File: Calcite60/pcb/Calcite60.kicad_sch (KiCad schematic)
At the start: 56 parts, among them J1 USB_C_Receptacle_USB2.0, J2 Conn_01x02, J3 Conn_01x02, J4 Conn_01x02, J4 Conn_02x05_Counter_Clockwise, J5 Conn_01x02, J6 Conn_01x04, Q1 AO3407, SW1 SW_DPDT_x2, U1 SRV05-4, U2 TP4054, U3 RT9013-33GB

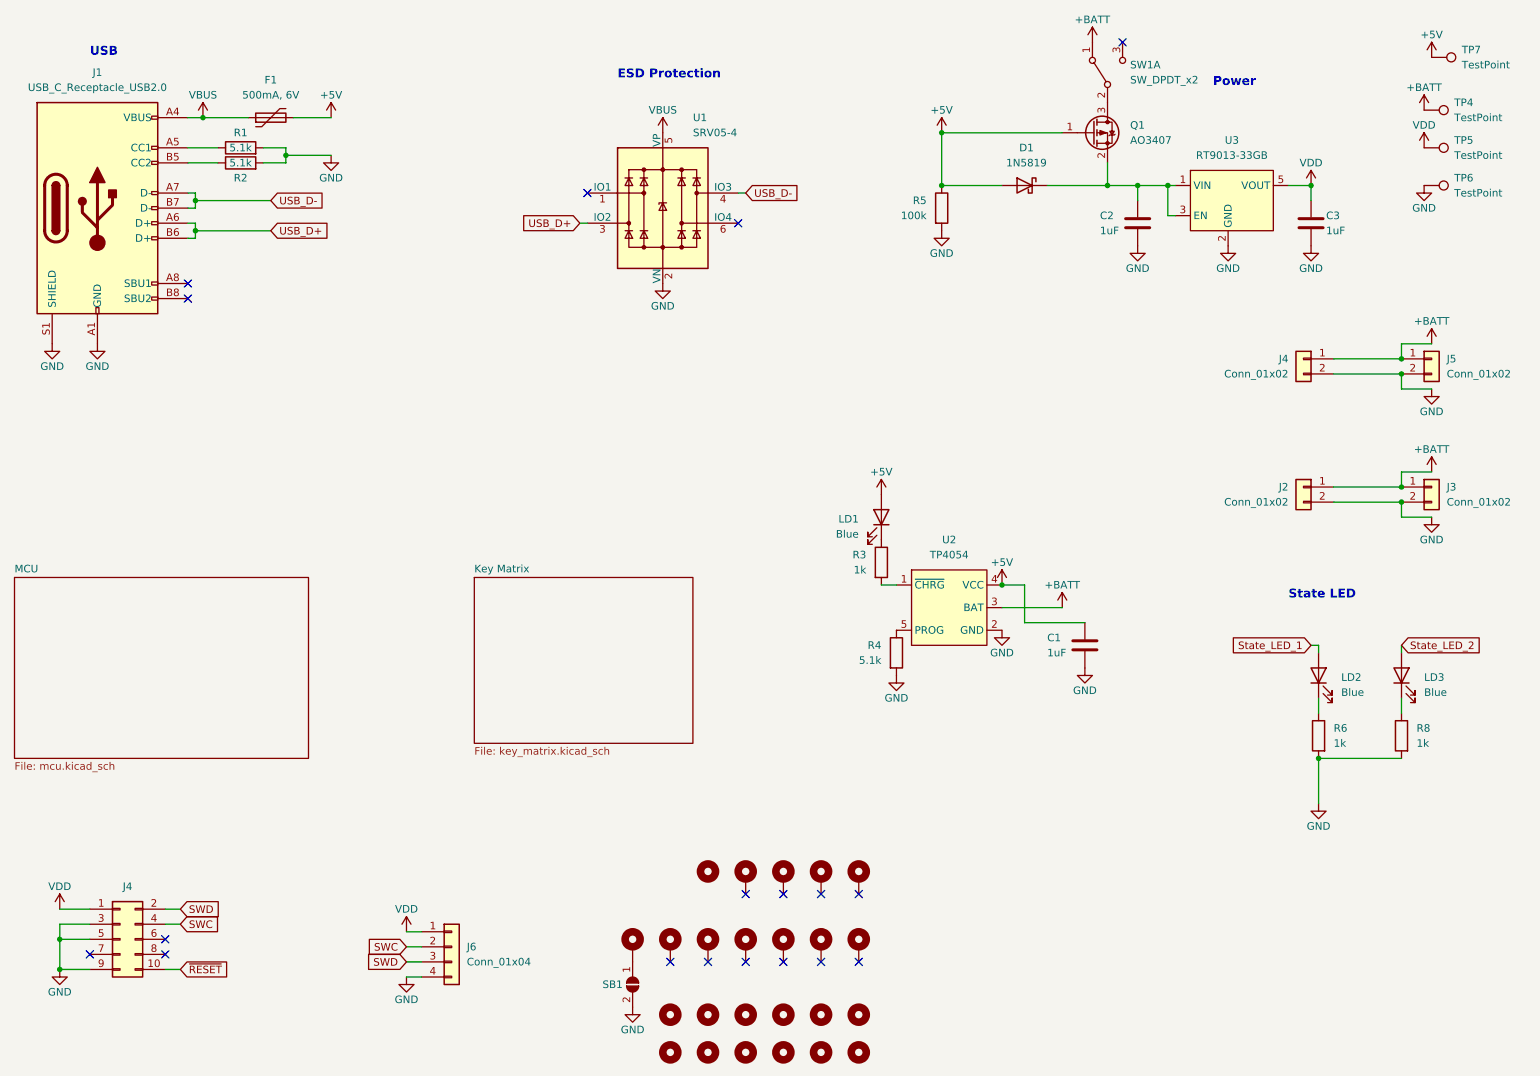
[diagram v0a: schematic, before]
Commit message: Update BOM
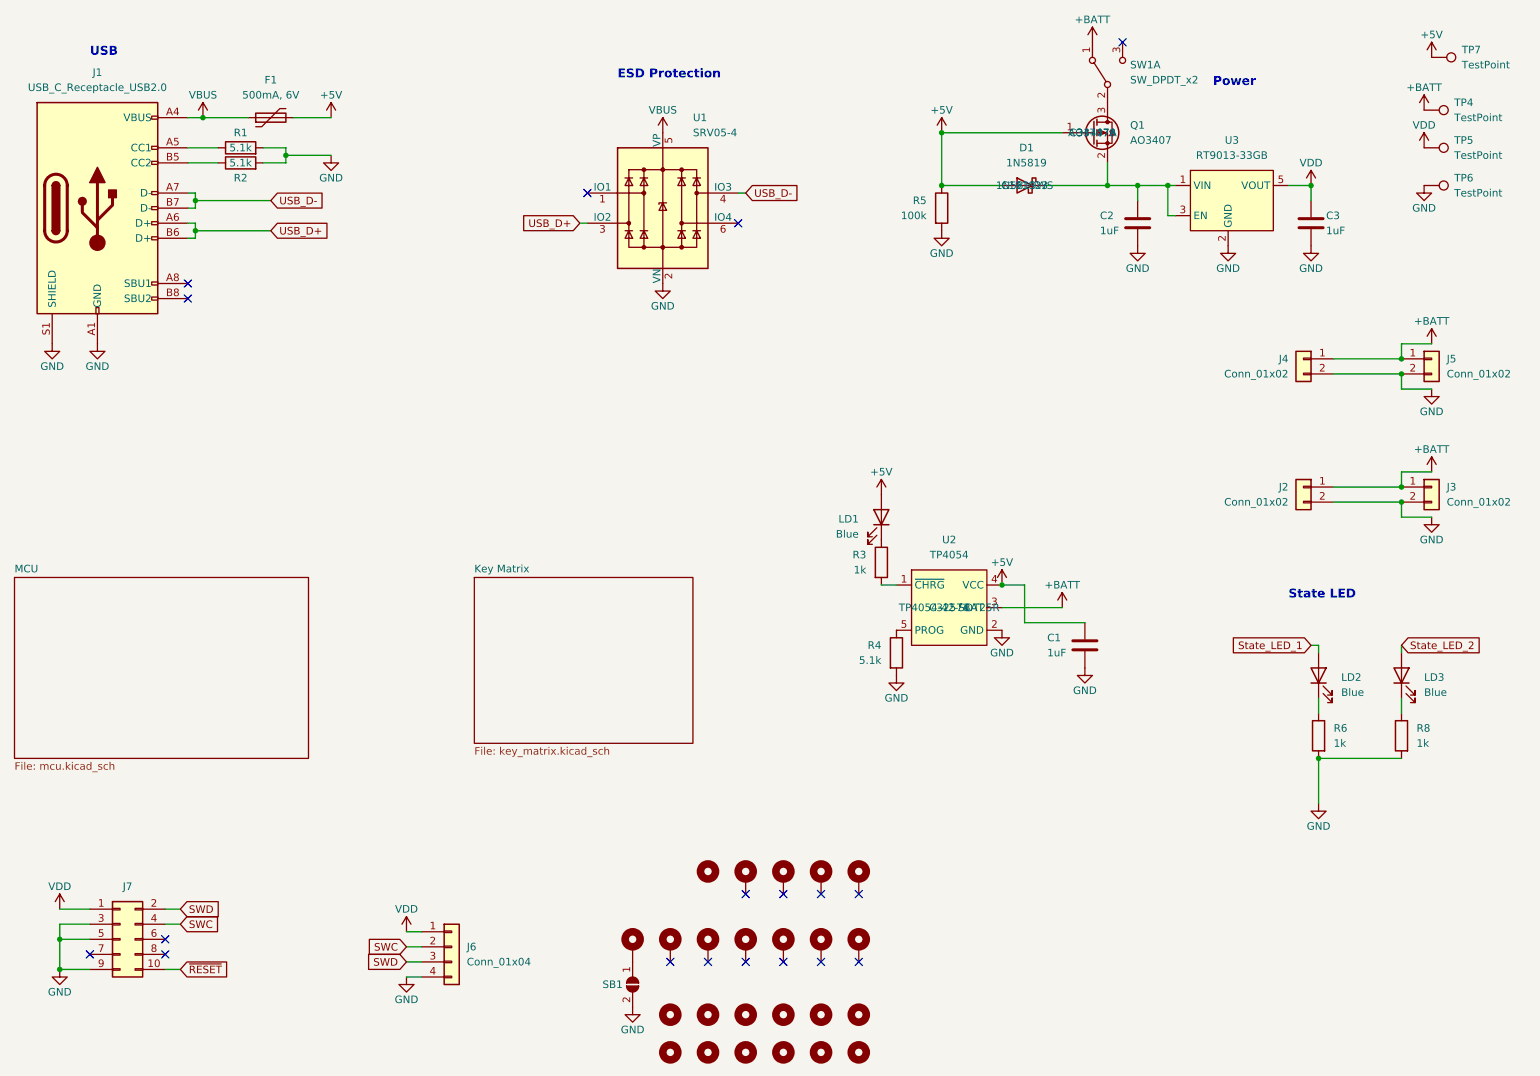
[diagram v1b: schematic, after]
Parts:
- C1, C2, C3: LCSC C52923 -> C15849; MFR. Part # CL05A105KA5NQNC -> CL10A105KB8NNNC
- D1: LCSC (none) -> C191023; MFR. Part # (none) -> 1N5819WS
- Q1: LCSC (none) -> C347478; MFR. Part # (none) -> AO3407A
- R1, R2: LCSC C25905 -> C23186; MFR. Part # 0402WGF5101TCE -> 0603WAF5101T5E
- R3, R6, R8: LCSC C11702 -> C21190; MFR. Part # 0402WGF1001TCE -> 0603WAF1001T5E
- R4: LCSC C11702 -> C23186; MFR. Part # 0402WGF1001TCE -> 0603WAF5101T5E
- R5: LCSC C11702 -> C25803; MFR. Part # 0402WGF1001TCE -> 0603WAF1003T5E
- U2: LCSC (none) -> C32574; MFR. Part # (none) -> TP4054-42-SOT25R
- renumbered J4 to J7
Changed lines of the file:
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@@
 (kicad_sch
-	(version 20231120)
+	(version 20250114)
 	(generator "eeschema")
-	(generator_version "8.0")
+	(generator_version "9.0")
 	(paper "A4")
 	(title_block
@@
 		(comment 2 "Kailh Choc V1 (PG1350) Low Profile Switches")
 	)
+	(text "ESD Protection"
+		(exclude_from_sim no)
+		(at 130.81 31.75 0)
+		(effects
+			(font
+				(size 1.5 1.5)
+				(thickness 0.3)
+				(bold yes)
+			)
+			(justify left bottom)
+		)
+	)
+	(text "State LED"
+		(exclude_from_sim no)
+		(at 243.84 119.38 0)
+		(effects
+			(font
+				(size 1.5 1.5)
+				(thickness 0.3)
+				(bold yes)
+			)
+			(justify left bottom)
+		)
+	)
+	(text "USB"
+		(exclude_from_sim no)
+		(at 41.91 27.94 0)
+		(effects
+			(font
+				(size 1.5 1.5)
+				(thickness 0.3)
+				(bold yes)
+			)
+			(justify left bottom)
+		)
+	)
+	(text "Power\n"
+		(exclude_from_sim no)
+		(at 231.14 33.02 0)
+		(effects
+			(font
+				(size 1.5 1.5)
+				(thickness 0.3)
+				(bold yes)
+			)
+			(justify left bottom)
+		)
+	)
 	(junction
 		(at 262.89 81.28)
@@
 		)
 	)
-	(text "ESD Protection"
-		(exclude_from_sim no)
-		(at 130.81 31.75 0)
-		(effects
-			(font
-				(size 1.5 1.5)
-				(thickness 0.3)
-				(bold yes)
-			)
-			(justify left bottom)
-		)
-	)
-	(text "State LED"
-		(exclude_from_sim no)
-		(at 243.84 119.38 0)
-		(effects
-			(font
-				(size 1.5 1.5)
-				(thickness 0.3)
-				(bold yes)
-			)
-			(justify left bottom)
-		)
-	)
-	(text "USB"
-		(exclude_from_sim no)
-		(at 41.91 27.94 0)
-		(effects
-			(font
-				(size 1.5 1.5)
-				(thickness 0.3)
-				(bold yes)
-			)
-			(justify left bottom)
-		)
-	)
-	(text "Power\n"
-		(exclude_from_sim no)
-		(at 231.14 33.02 0)
-		(effects
-			(font
-				(size 1.5 1.5)
-				(thickness 0.3)
-				(bold yes)
-			)
-			(justify left bottom)
-		)
-	)
 	(global_label "SWC"
 		(shape input)
@@
 			)
 		)
-		(property "MFR. Part #" "0402WGF1001TCE "
+		(property "MFR. Part #" "0603WAF1001T5E"
 			(at 262.89 142.24 0)
 			(effects
@@
 			)
 		)
-		(property "LCSC" "C11702"
+		(property "LCSC" "C21190"
 			(at 262.89 142.24 0)
 			(effects
@@
 			)
 		)
-		(property "MFR. Part #" "0402WGF1001TCE "
+		(property "MFR. Part #" "0603WAF5101T5E"
 			(at 177.8 128.27 0)
 			(effects
@@
 			)
 		)
-		(property "LCSC" "C11702"
+		(property "LCSC" "C23186"
 			(at 177.8 128.27 0)
 			(effects
@@
 		(on_board yes)
 		(dnp no)
-		(property "Reference" "J4"
+		(property "Reference" "J7"
 			(at 48.26 167.64 0)
 			(effects
@@
 		(on_board yes)
 		(dnp no)
-		(property "Reference" "#PWR018"
+		(property "Reference" "#PWR038"
 			(at 36.83 187.96 0)
 			(effects
@@
 			)
 		)
-		(property "MFR. Part #" "0402WGF1001TCE "
+		(property "MFR. Part #" "0603WAF1001T5E"
 			(at 248.92 142.24 0)
 			(effects
@@
 			)
 		)
-		(property "LCSC" "C11702"
+		(property "LCSC" "C21190"
 			(at 248.92 142.24 0)
 			(effects
@@
 			)
 		)
-		(property "MFR. Part #" "0402WGF5101TCE"
+		(property "MFR. Part #" "0603WAF5101T5E"
 			(at 67.31 45.72 0)
 			(effects
@@
 			)
 		)
-		(property "LCSC" "C25905"
+		(property "LCSC" "C23186"
 			(at 67.31 45.72 0)
 			(effects
@@
 			)
 		)
-		(property "MFR. Part #" "CL05A105KA5NQNC"
+		(property "MFR. Part #" "CL10A105KB8NNNC"
 			(at 209.55 127 0)
 			(effects
@@
 			)
 		)
-		(property "LCSC" "C52923"
+		(property "LCSC" "C15849"
 			(at 209.55 127 0)
 			(effects
@@
 			)
 		)
+		(property "LCSC" "C347478"
+			(at 210.82 40.64 0)
+			(effects
+				(font
+					(size 1.27 1.27)
+				)
+			)
+		)
+		(property "MFR. Part #" "AO3407A"
+			(at 210.82 40.64 0)
+			(effects
+				(font
+					(size 1.27 1.27)
+				)
+			)
+		)
 		(pin "1"
 		)
@@
 			)
 		)
-		(property "MFR. Part #" "0402WGF1001TCE "
+		(property "MFR. Part #" "0603WAF1003T5E"
 			(at 185.42 53.34 0)
 			(effects
@@
 			)
 		)
-		(property "LCSC" "C11702"
+		(property "LCSC" "C25803"
 			(at 185.42 53.34 0)
 			(effects
@@
 			)
 		)
+		(property "LCSC" "C191023"
+			(at 199.39 49.53 0)
+			(effects
+				(font
+					(size 1.27 1.27)
+				)
+			)
+		)
+		(property "MFR. Part #" "1N5819WS"
+			(at 199.39 49.53 0)
+			(effects
+				(font
+					(size 1.27 1.27)
+				)
+			)
+		)
 		(pin "1"
 		)
@@
 			)
 		)
-		(property "MFR. Part #" "CL05A105KA5NQNC"
+		(property "MFR. Part #" "CL10A105KB8NNNC"
 			(at 247.65 55.88 0)
 			(effects
@@
 			)
 		)
-		(property "LCSC" "C52923"
+		(property "LCSC" "C15849"
 			(at 247.65 55.88 0)
 			(effects
@@
 			)
 		)
-		(property "MFR. Part #" "0402WGF1001TCE "
+		(property "MFR. Part #" "0603WAF1001T5E"
 			(at 175.26 113.03 0)
 			(effects
@@
 			)
 		)
-		(property "LCSC" "C11702"
+		(property "LCSC" "C21190"
 			(at 175.26 113.03 0)
 			(effects
@@
 			)
 		)
-		(property "MFR. Part #" "0402WGF5101TCE"
+		(property "MFR. Part #" "0603WAF5101T5E"
 			(at 67.31 43.18 0)
 			(effects
@@
 			)
 		)
-		(property "LCSC" "C25905"
+		(property "LCSC" "C23186"
 			(at 67.31 43.18 0)
 			(effects
@@
 			)
 		)
+		(property "LCSC" "C32574"
+			(at 186.69 120.65 0)
+			(effects
+				(font
+					(size 1.27 1.27)
+				)
+			)
+		)
+		(property "MFR. Part #" "TP4054-42-SOT25R"
+			(at 186.69 120.65 0)
+			(effects
+				(font
+					(size 1.27 1.27)
+				)
+			)
+		)
 		(pin "1"
 		)
@@
 			)
 		)
-		(property "MFR. Part #" "CL05A105KA5NQNC"
+		(property "MFR. Part #" "CL10A105KB8NNNC"
 			(at 218.44 55.88 0)
 			(effects
@@
 			)
 		)
-		(property "LCSC" "C52923"
+		(property "LCSC" "C15849"
 			(at 218.44 55.88 0)
 			(effects
@@
 		(at 29.21 115.57)
 		(size 49.53 30.48)
+		(exclude_from_sim no)
+		(in_bom yes)
+		(on_board yes)
+		(dnp no)
 		(fields_autoplaced yes)
 		(stroke
@@
 		(at 106.68 115.57)
 		(size 36.83 27.94)
+		(exclude_from_sim no)
+		(in_bom yes)
+		(on_board yes)
+		(dnp no)
 		(fields_autoplaced yes)
 		(stroke
@@
 		)
 	)
+	(embedded_fonts no)
 )
